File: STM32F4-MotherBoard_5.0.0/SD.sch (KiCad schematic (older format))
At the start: 1 part, among them CON1 SD_Card

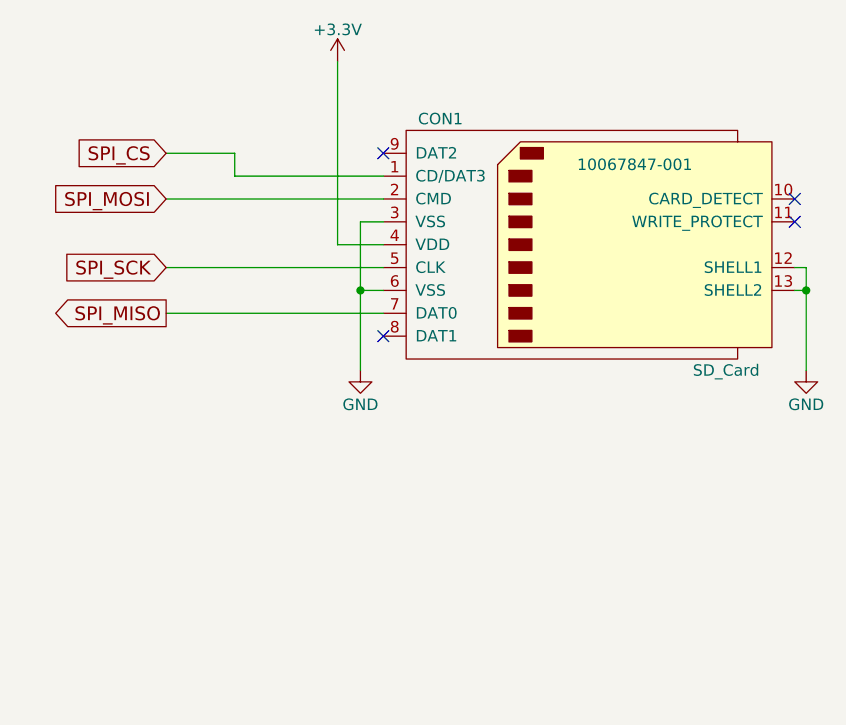
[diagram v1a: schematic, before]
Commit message: replace project
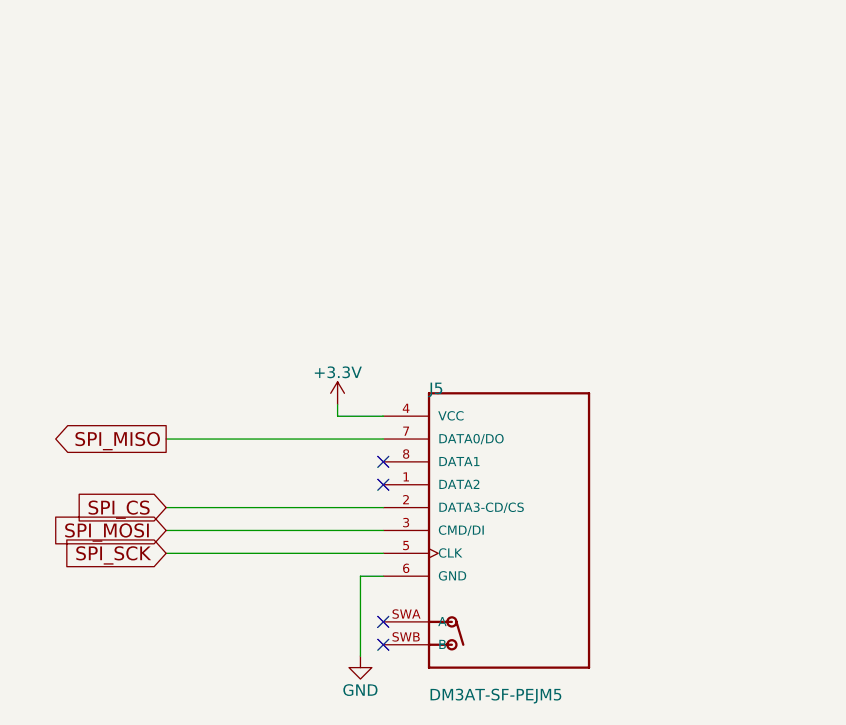
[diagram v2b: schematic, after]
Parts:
- removed CON1: SD_Card, 10067847-001, symbol SD_Card
- added J5: DM3AT-SF-PEJM5, DM3AT-SF-PEJM5:HRS_DM3AT-SF-PEJM5, symbol DM3AT-SF-PEJM5
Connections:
- net +3V3: now also J5.4 (VCC)
- net GND: now also J5.6 (GND)
- net SPI_CS: now also J5.2 (DATA3-CD/CS)
- net SPI_MISO: now also J5.7 (DATA0/DO)
- net SPI_MOSI: now also J5.3 (CMD/DI)
- net SPI_SCK: now also J5.5 (CLK)
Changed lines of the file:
@@
 LIBS:STM32F4-MotherBoard_3.0.0-cache
 LIBS:STM32F4-MotherBoard_5.0.0-cache
+LIBS:DM3AT-SF-PEJM5
 EELAYER 25 0
 EELAYER END
@@
 Comment4 ""
 $EndDescr
-Text GLabel 4350 3350 0    60   Input ~ 0
+Text GLabel 4350 4600 0    60   Input ~ 0
 SPI_SCK
-Text GLabel 4350 3050 0    60   Input ~ 0
+Text GLabel 4350 4500 0    60   Input ~ 0
 SPI_MOSI
-Text GLabel 4350 3550 0    60   Output ~ 0
+Text GLabel 4350 4100 0    60   Output ~ 0
 SPI_MISO
+Wire Wire Line
+	5300 4100 4350 4100
+Wire Wire Line
+	4350 4500 5300 4500
+Wire Wire Line
+	4350 4600 5300 4600
+Wire Wire Line
+	4350 4400 5300 4400
 $Comp
-L SD_Card CON1
-U 1 1 58A2FDC9
-P 6200 3250
-F 0 "CON1" H 5550 3800 50  0000 C CNN
-F 1 "SD_Card" H 6800 2700 50  0000 C CNN
-F 2 "10067847-001" H 6400 3600 50  0000 C CNN
-F 3 "" H 6200 3250 50  0000 C CNN
-	1    6200 3250
+L GND #PWR072
+U 1 1 58A2FE1C
+P 5200 5050
+F 0 "#PWR072" H 5200 4800 50  0001 C CNN
+F 1 "GND" H 5200 4900 50  0000 C CNN
+F 2 "" H 5200 5050 50  0000 C CNN
+F 3 "" H 5200 5050 50  0000 C CNN
+	1    5200 5050
+	1    0    0    -1
+$EndComp
+$Comp
+L +3.3V #PWR073
+U 1 1 58A2FE3B
+P 5100 3950
+F 0 "#PWR073" H 5100 3800 50  0001 C CNN
+F 1 "+3.3V" H 5100 4090 50  0000 C CNN
+F 2 "" H 5100 3950 50  0000 C CNN
+F 3 "" H 5100 3950 50  0000 C CNN
+	1    5100 3950
 	1    0    0    -1
 $EndComp
 Wire Wire Line
-	5300 3550 4350 3550
+	5100 4000 5300 4000
 Wire Wire Line
-	4350 3050 5300 3050
-Wire Wire Line
-	4350 3350 5300 3350
-Wire Wire Line
-	4650 2950 5300 2950
+	5300 4700 5200 4700
+NoConn ~ 5300 4200
+Text GLabel 4350 4400 0    60   Input ~ 0
+SPI_CS
+NoConn ~ 5300 4300
 $Comp
-L GND #PWR072
-U 1 1 58A2FE1C
-P 5200 3800
-F 0 "#PWR072" H 5200 3550 50  0001 C CNN
-F 1 "GND" H 5200 3650 50  0000 C CNN
-F 2 "" H 5200 3800 50  0000 C CNN
-F 3 "" H 5200 3800 50  0000 C CNN
-	1    5200 3800
+L DM3AT-SF-PEJM5 J5
+U 1 1 58DE04A7
+P 5500 4500
+F 0 "J5" H 5500 5120 50  0000 L CNN
+F 1 "DM3AT-SF-PEJM5" H 5500 3780 50  0000 L CNN
+F 2 "DM3AT-SF-PEJM5:HRS_DM3AT-SF-PEJM5" H 5500 4500 50  0001 L CNN
+F 3 "DM3AT-SF-PEJM5" H 5500 4500 50  0001 L CNN
+F 4 "Good" H 5500 4500 50  0001 L CNN "Availability"
+F 5 "DM3 Series 8 Position Right Angle SMT Push Push Ejection MicroSD Card Connector" H 5500 4500 50  0001 L CNN "Description"
+F 6 "None" H 5500 4500 50  0001 L CNN "Package"
+F 7 "Hirose" H 5500 4500 50  0001 L CNN "MF"
+F 8 "1.96 USD" H 5500 4500 50  0001 L CNN "Price"
+	1    5500 4500
 	1    0    0    -1
 $EndComp
 Wire Wire Line
-	5300 3150 5200 3150
-$Comp
-L +3.3V #PWR073
-U 1 1 58A2FE3B
-P 5100 2450
-F 0 "#PWR073" H 5100 2300 50  0001 C CNN
-F 1 "+3.3V" H 5100 2590 50  0000 C CNN
-F 2 "" H 5100 2450 50  0000 C CNN
-F 3 "" H 5100 2450 50  0000 C CNN
-	1    5100 2450
-	1    0    0    -1
-$EndComp
+	5200 4700 5200 5050
 Wire Wire Line
-	5100 2450 5100 3250
-Wire Wire Line
-	5100 3250 5300 3250
-Wire Wire Line
-	5300 3450 5200 3450
-Connection ~ 5200 3450
-NoConn ~ 5300 2850
-NoConn ~ 5300 3650
-NoConn ~ 7100 3050
-NoConn ~ 7100 3150
-Wire Wire Line
-	7100 3350 7150 3350
-Wire Wire Line
-	7150 3350 7150 3800
-Wire Wire Line
-	7150 3450 7100 3450
-Connection ~ 7150 3450
-$Comp
-L GND #PWR074
-U 1 1 58A2FEA7
-P 7150 3800
-F 0 "#PWR074" H 7150 3550 50  0001 C CNN
-F 1 "GND" H 7150 3650 50  0000 C CNN
-F 2 "" H 7150 3800 50  0000 C CNN
-F 3 "" H 7150 3800 50  0000 C CNN
-	1    7150 3800
-	1    0    0    -1
-$EndComp
-Wire Wire Line
-	5200 3150 5200 3800
-Wire Wire Line
-	4650 2950 4650 2850
-Wire Wire Line
-	4650 2850 4350 2850
-Text GLabel 4350 2850 0    60   Input ~ 0
-SPI_CS
+	5100 4000 5100 3950
+NoConn ~ 5300 4900
+NoConn ~ 5300 5000
 $EndSCHEMATC
